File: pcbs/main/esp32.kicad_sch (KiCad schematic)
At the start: 1 part, among them U1 ESP32-DEVKITC-32U

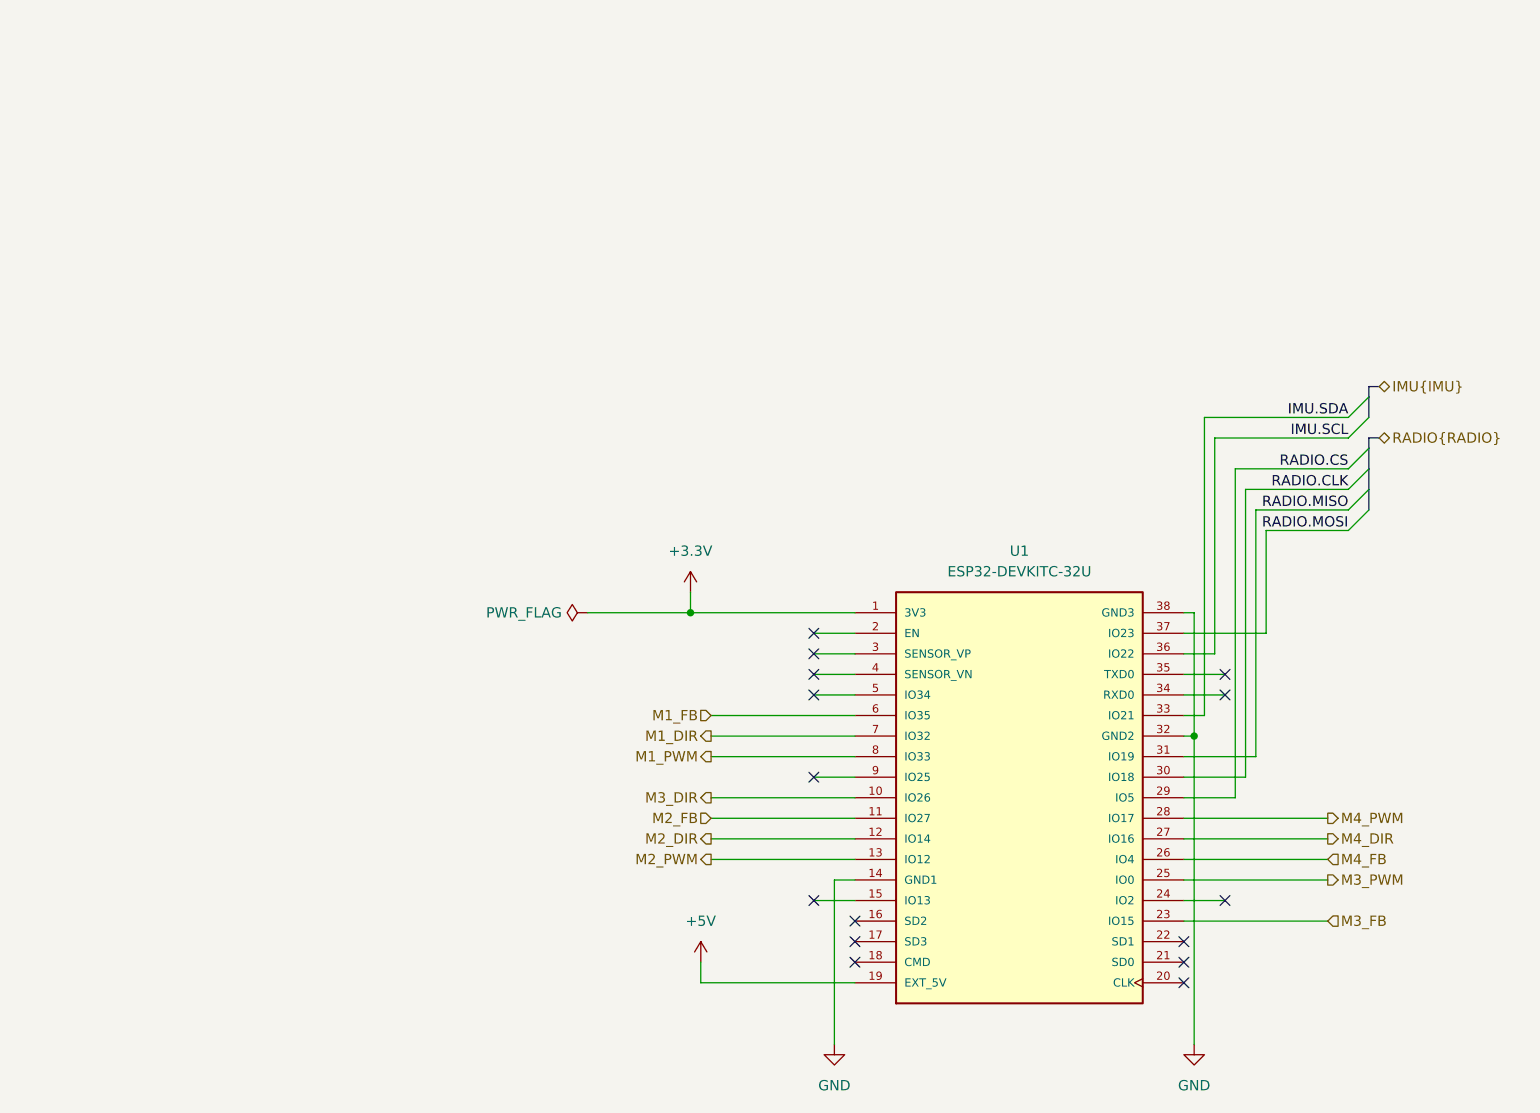
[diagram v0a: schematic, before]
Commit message: Edits for custom board
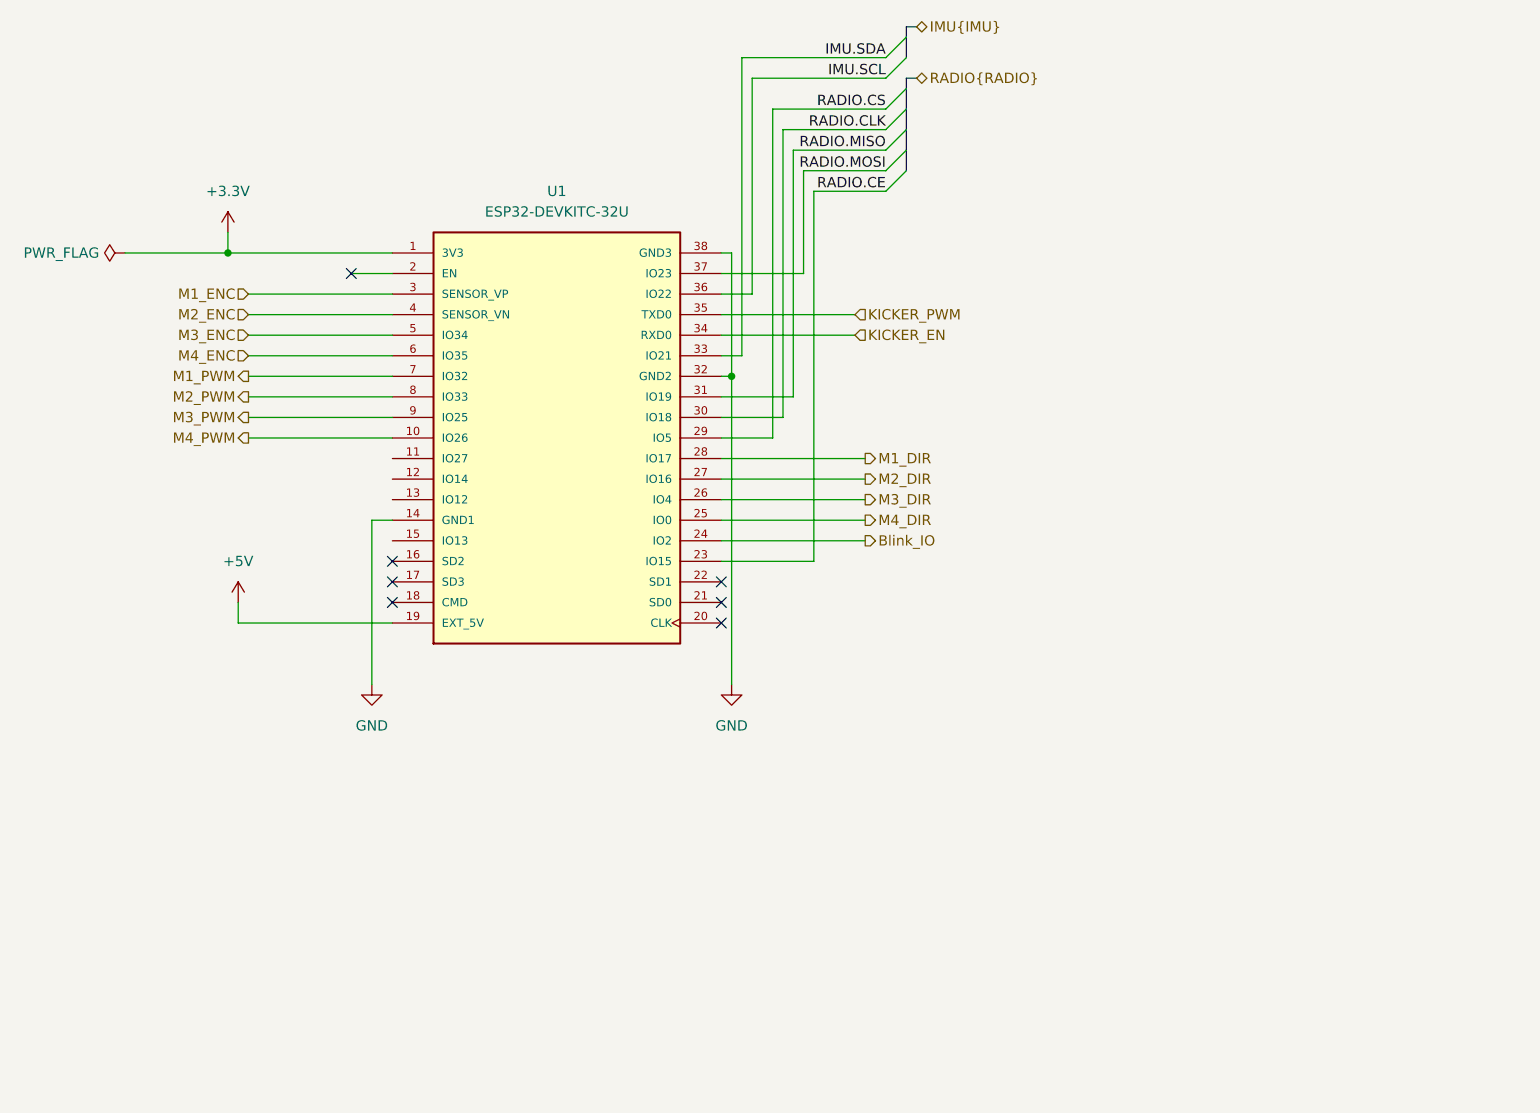
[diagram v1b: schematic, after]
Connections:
- net M4_FB is gone; now on net M3_DIR: U1.26 (IO4)
- net M1_DIR: now also U1.28 (IO17); no longer U1.7 (IO32)
- net M1_PWM: now also U1.7 (IO32); no longer U1.8 (IO33)
- net M2_DIR: now also U1.27 (IO16); no longer U1.12 (IO14)
- net M2_PWM: now also U1.8 (IO33); no longer U1.13 (IO12)
- net M3_DIR: no longer U1.10 (IO26)
- net M3_PWM: now also U1.9 (IO25); no longer U1.25 (IO0)
- net M4_DIR: now also U1.25 (IO0); no longer U1.27 (IO16)
- net M4_PWM: now also U1.10 (IO26); no longer U1.28 (IO17)
- net Blink_IO: now reaches U1.24 (IO2)
- net M1_ENC: now reaches U1.3 (SENSOR_VP)
- net KICKER_EN: now reaches U1.34 (RXD0)
- net KICKER_PWM: now reaches U1.35 (TXD0)
- net M2_ENC: now reaches U1.4 (SENSOR_VN)
- net M3_ENC: now reaches U1.5 (IO34)
- net M1_FB renamed M4_ENC
- net M2_FB: no longer names the net of U1.11 (IO27)
- net M3_FB renamed RADIO.CE
- no-connect marks 15 -> 7
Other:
- moved on the sheet: U1
